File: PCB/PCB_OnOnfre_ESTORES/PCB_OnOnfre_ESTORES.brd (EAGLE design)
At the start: 44 x 41.7 mm, 28 parts, among them J1 9PIN 2.54MM, J3Y S8050, J7 8p, K1 OMRON-G3MB-202P-SSR2, K2 OMRON-G3MB-202P-SSR2, U2 esp12

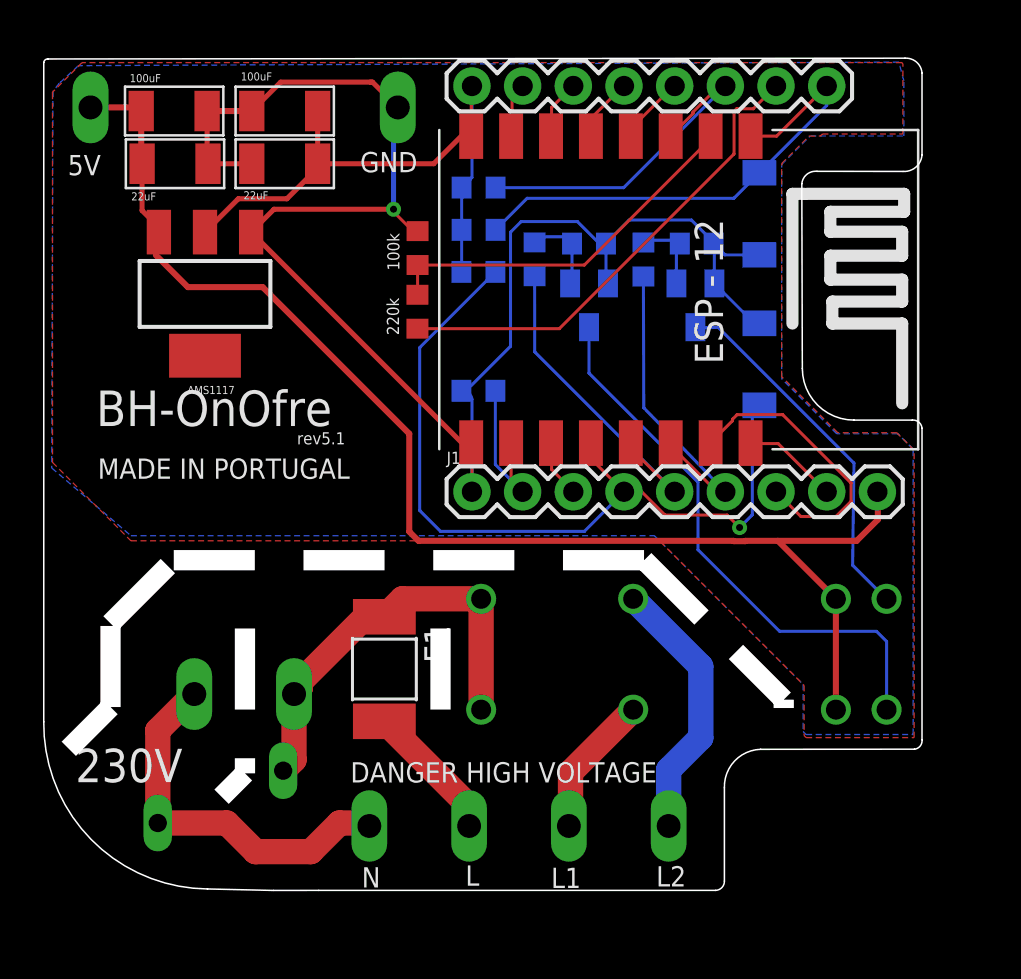
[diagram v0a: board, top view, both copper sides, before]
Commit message: Estores Rev1
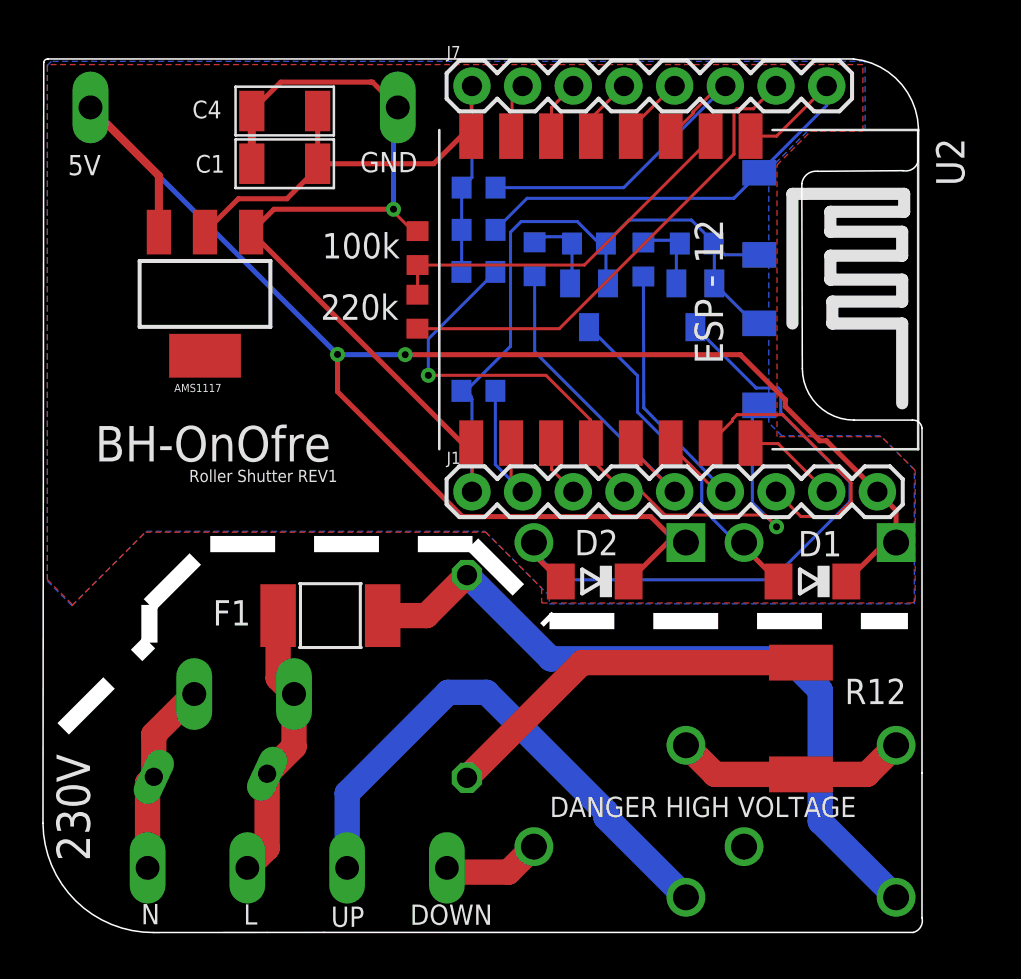
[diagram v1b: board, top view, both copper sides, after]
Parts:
- removed C2: 22uF, Seeed-Capacitor:C1206
- removed C3: 100uF, Seeed-Capacitor:C1206
- added C6: (no value), rcl:C102-043X133
- added D1, D2: 1N4148, diode:SOD80C
- added R12: (no value), resistor:R2512
- C1: value 22uF -> 1NF
- C4: value 100uF -> 1NF
- K1, K2: value OMRON-G3MB-202P-SSR2 -> G5Q-1-DC12; device Omron G3MB 202p SSR:OMRON-G3MB-202P-SSR -> G5Q-1-DC12:RELAY_G5Q-1-DC12
- R5: value S07K230 -> VARISTORS07K230; device VARISTORESBH:S07K230 -> varistor:S07K230
- moved X1 11.3 mm to (13.4, 4.52)
- moved K2 8.87 mm to (28.9, 13.1), turned to 270 degrees
- moved K1 4.18 mm to (39.4, 13.1), turned to 270 degrees
- moved F1 3.81 mm to (15.1, 18.4), turned to 180 degrees
- moved R5 1.20 mm to (9.04, 10.4), turned to 295 degrees
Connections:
- removed net LINE_ONE_OUT: K1.2, X1.3
- removed net LINE_TWO_OUT: K2.2, X1.4
- removed net N$2: F1.2, X1.2
- new net LINE_DOWN_OUT: K2.4, X1.4
- new net LINE_IN_FUSED: C6.1, F1.1, K1.3
- new net LINE_UP_OUT: K2.3, X1.3
- new net N$3: K1.2, K2.2, R12.2
- new net N$5: C6.2, R12.1
- net GND: no longer C2.2, C3.2
- net LINE_L: now also F1.2, X1.2; no longer F1.1, K1.1, K2.1
- net N$1: now also D1.A, K1.5; no longer K1.4
- net N$9: now also D2.A, K2.5; no longer K2.4
- net VCC: now also D1.C, D2.C, K1.1, K2.1; no longer C2.1, C3.1, K1.3, K2.3
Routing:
- net LINE_IN_FUSED: track 0.00 -> 37.1 mm
- net LINE_UP_OUT: track 0.00 -> 27.2 mm
- net VCC: track 67.4 -> 87.7 mm, vias 0 -> 2
- net N$5: track 0.00 -> 19.1 mm
- net N$9: track 18.3 -> 33.6 mm
- net LINE_TWO_OUT: track 13.5 -> 0.00 mm
- net N$3: track 0.00 -> 11.7 mm
- net N$1: track 28.2 -> 16.9 mm
- net NEUTRAL_IN: track 19.1 -> 9.68 mm
- net LINE_L: track 21.1 -> 13.9 mm
- net LINE_ONE_OUT: track 7.16 -> 0.00 mm
- net N$2: track 7.00 -> 0.00 mm
- net GPIO0: track 41.4 -> 35.6 mm, vias 1 -> 2
- net LINE_DOWN_OUT: track 0.00 -> 4.98 mm
- net GND: track 84.6 -> 80.1 mm
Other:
- board size 44 x 41.7 mm -> 44.1 x 43.8 mm
- board text added: "DOWN"
- board text added: "Roller Shutter REV1"
- board text added: "UP"
- board text removed: "HLK-PM01"
- board text removed: "L1"
- board text removed: "L2"
- board text removed: "MADE IN PORTUGAL"
- board text removed: "rev5.1"
